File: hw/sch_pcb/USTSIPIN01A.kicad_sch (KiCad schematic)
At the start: 53 parts, among them M1 HOLE, M2 HOLE, M3 HOLE, M4 HOLE, M5 BMI-S-210-F, M6 BMI-S-210-F, M7 BMI-S-210-F, M8 BMI-S-204-F, U1 OPA2314, U2 OPA2314, U3 ISL21080DIH312Z-TK 1V25, U4 TS7211, U5 TS5A4594

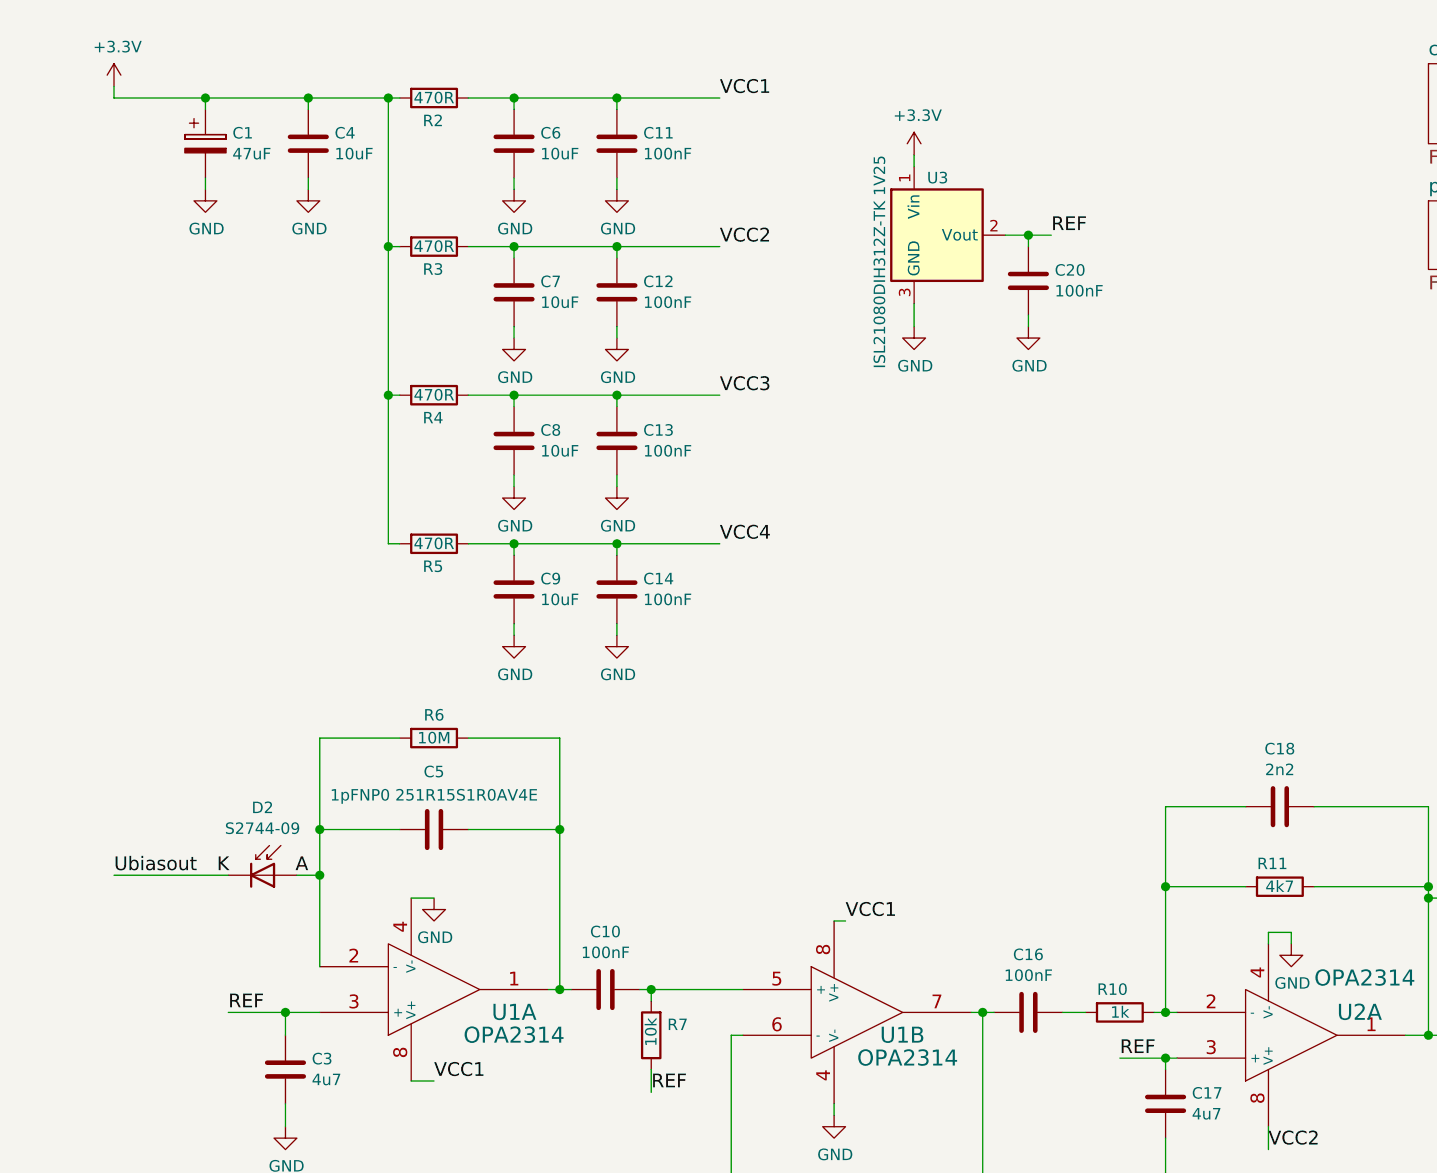
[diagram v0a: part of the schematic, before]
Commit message: Edit schema
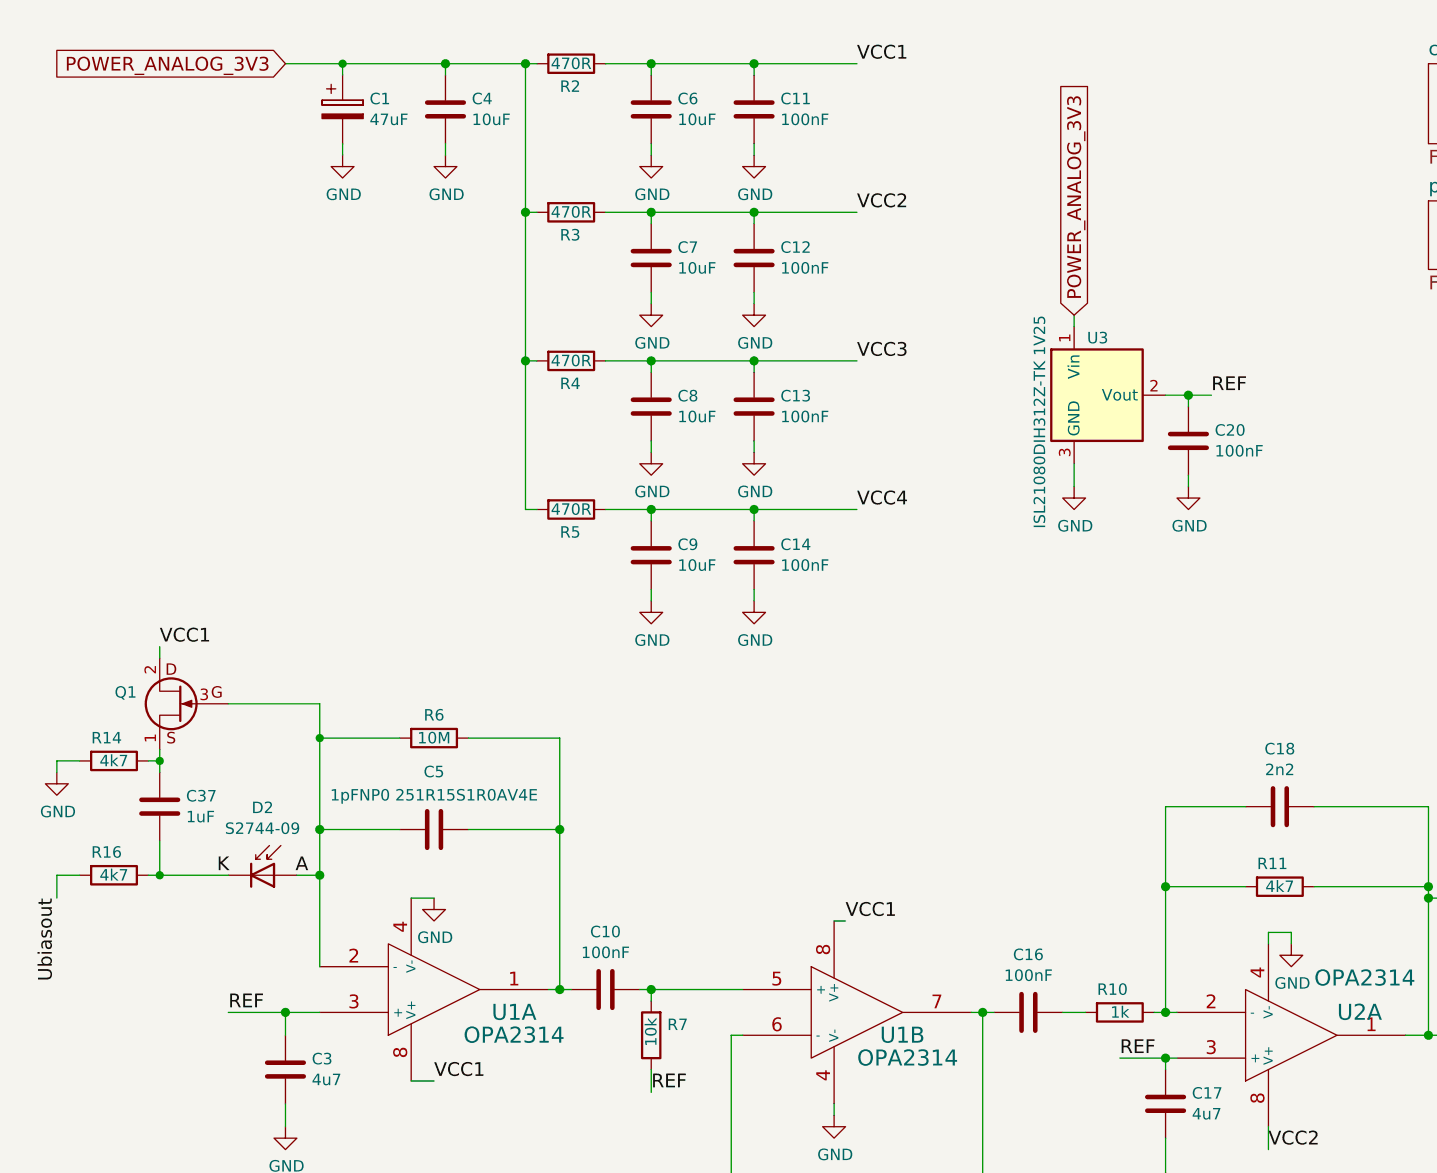
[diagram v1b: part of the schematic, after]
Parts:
- added C37: 1uF, Mlab_R:SMD-0805, symbol Device:C
- added Q1: (no value), symbol MLAB_T:Q_NJFET_SDG
- added R14, R16: 4k7, Mlab_R:SMD-0805, symbol Device:R
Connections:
- net A: now also Q1.3 (G)
- net GND: now also R14.2
- net K: now also C37.2, R16.1; no longer C24.1, R22.1
- net VCC1: now also Q1.2 (D)
- net +3V3 renamed POWER_ANALOG_3V3
- new net: C37.1, Q1.1 (S), R14.1
- new net Ubiasout: C24.1, R16.2, R22.1
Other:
- moved on the sheet: C1, C11, C12, C13, C14, C20, C4, C6, C7, C8, C9, R2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
